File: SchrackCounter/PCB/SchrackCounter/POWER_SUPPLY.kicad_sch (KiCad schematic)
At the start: 7 parts, among them J1 Conn_01x02_Pin, U1 LM1084-3.3

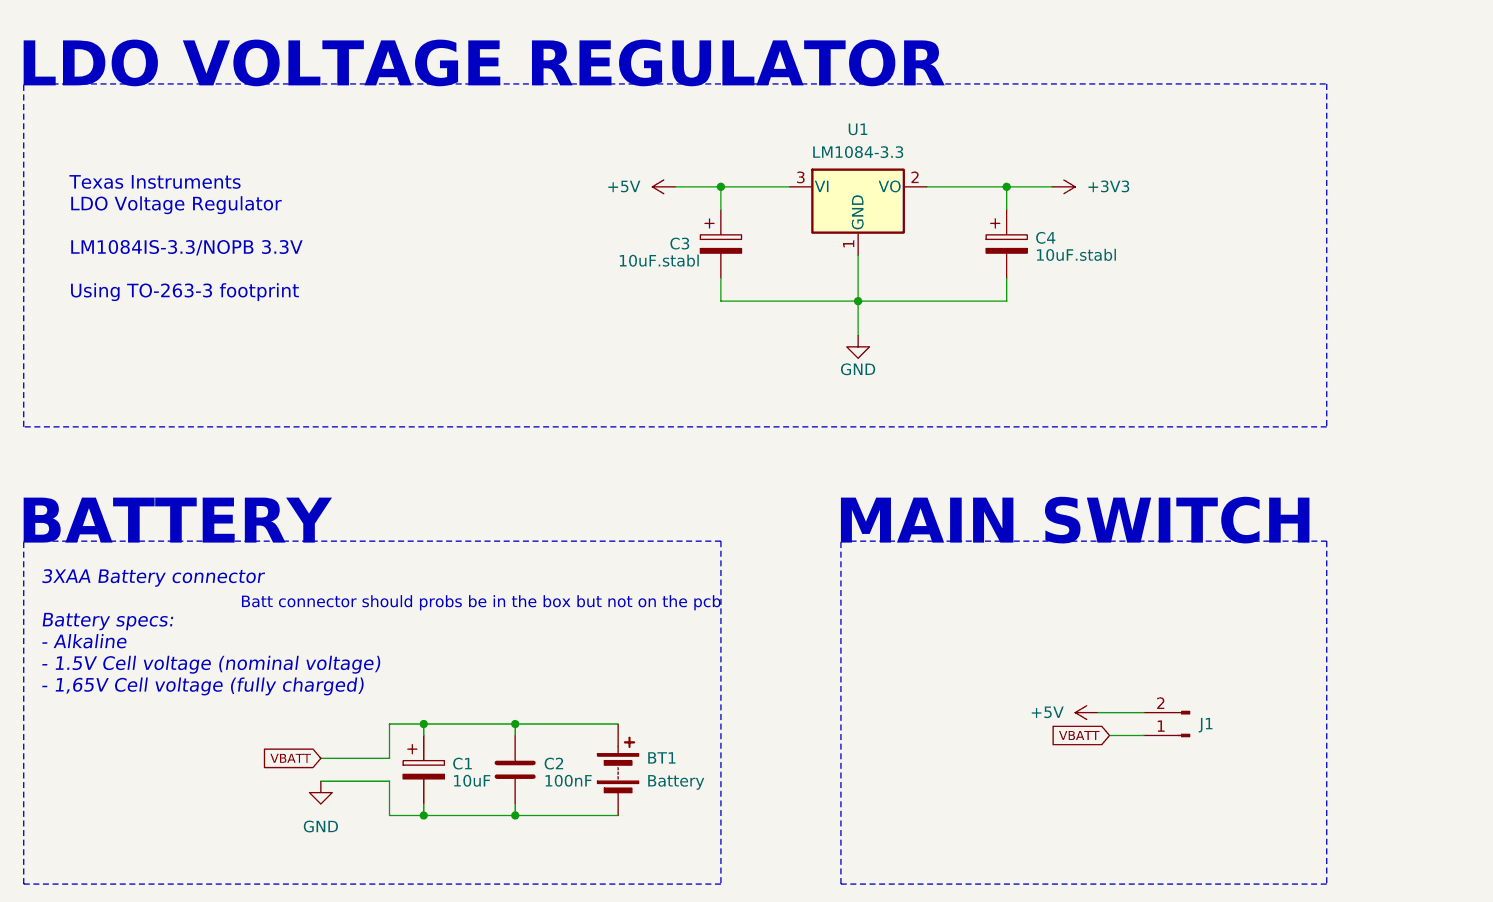
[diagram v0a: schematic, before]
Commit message: SchrackCounter
PCB Finished
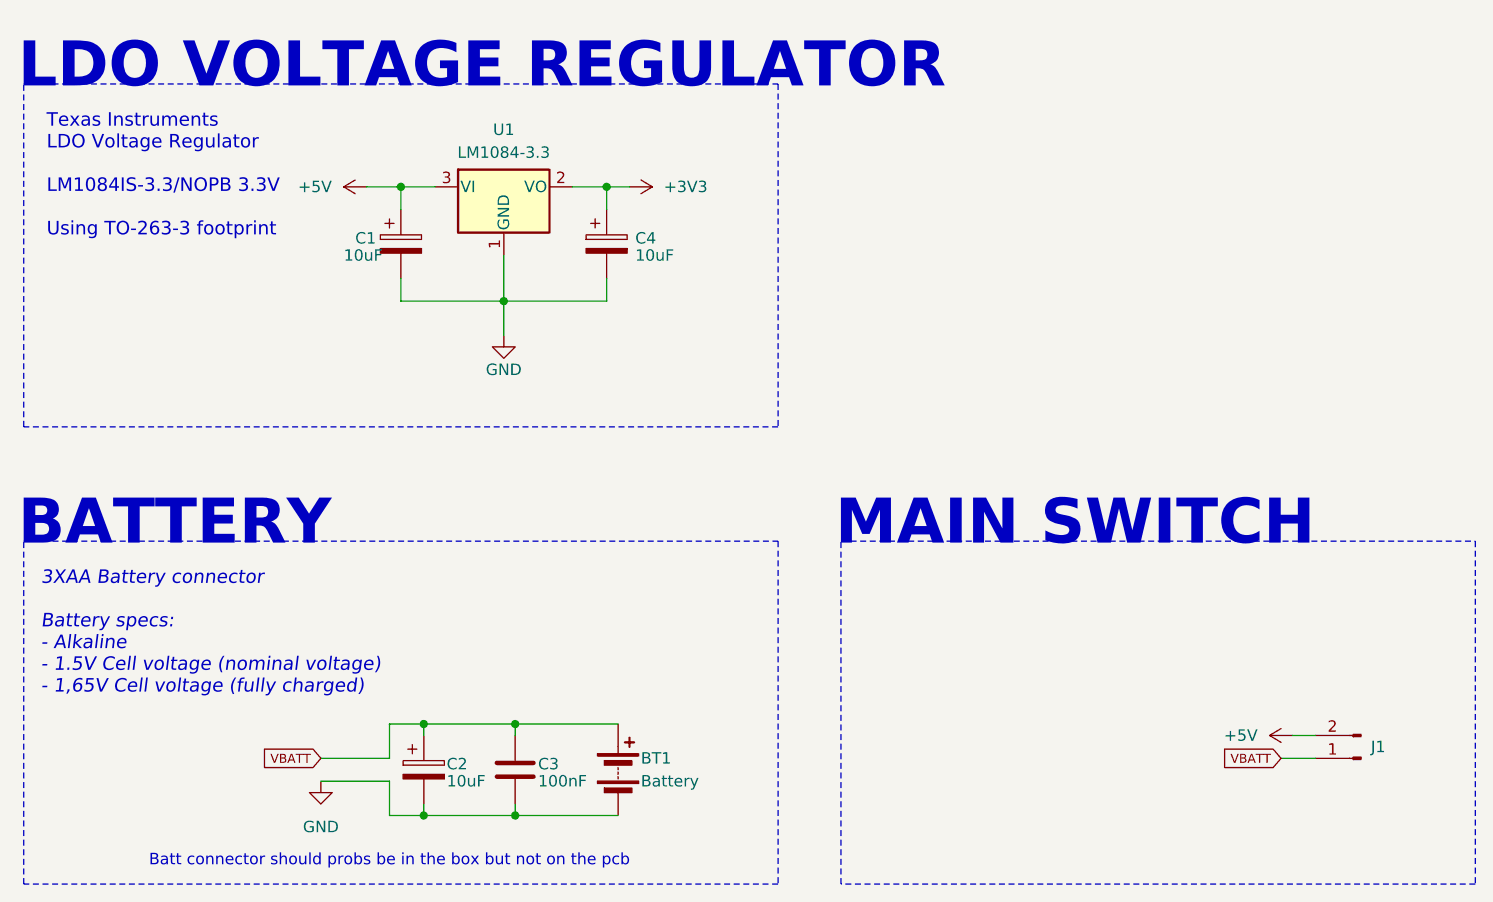
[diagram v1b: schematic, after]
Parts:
- C1: renamed from C3; value 10uF.stabl -> 10uF
- C4: value 10uF.stabl -> 10uF
- renumbered C1 to C2, C2 to C3
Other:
- moved on the sheet: C1, C4, J1, U1
